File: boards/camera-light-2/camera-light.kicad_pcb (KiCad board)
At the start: 2 copper layers, 10 x 9 mm, 3 parts, among them P1 CONN_01X02

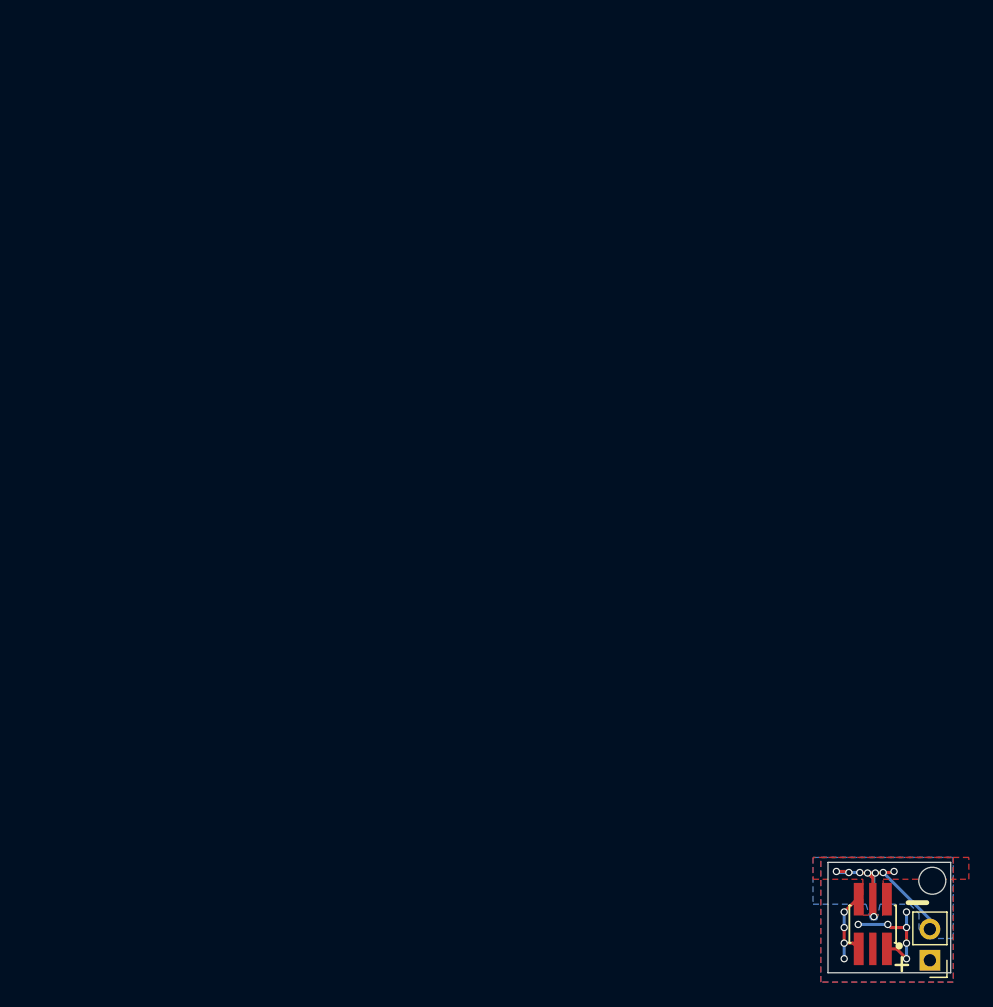
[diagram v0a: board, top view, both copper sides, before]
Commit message: [camera-light-2] export schematic and layout
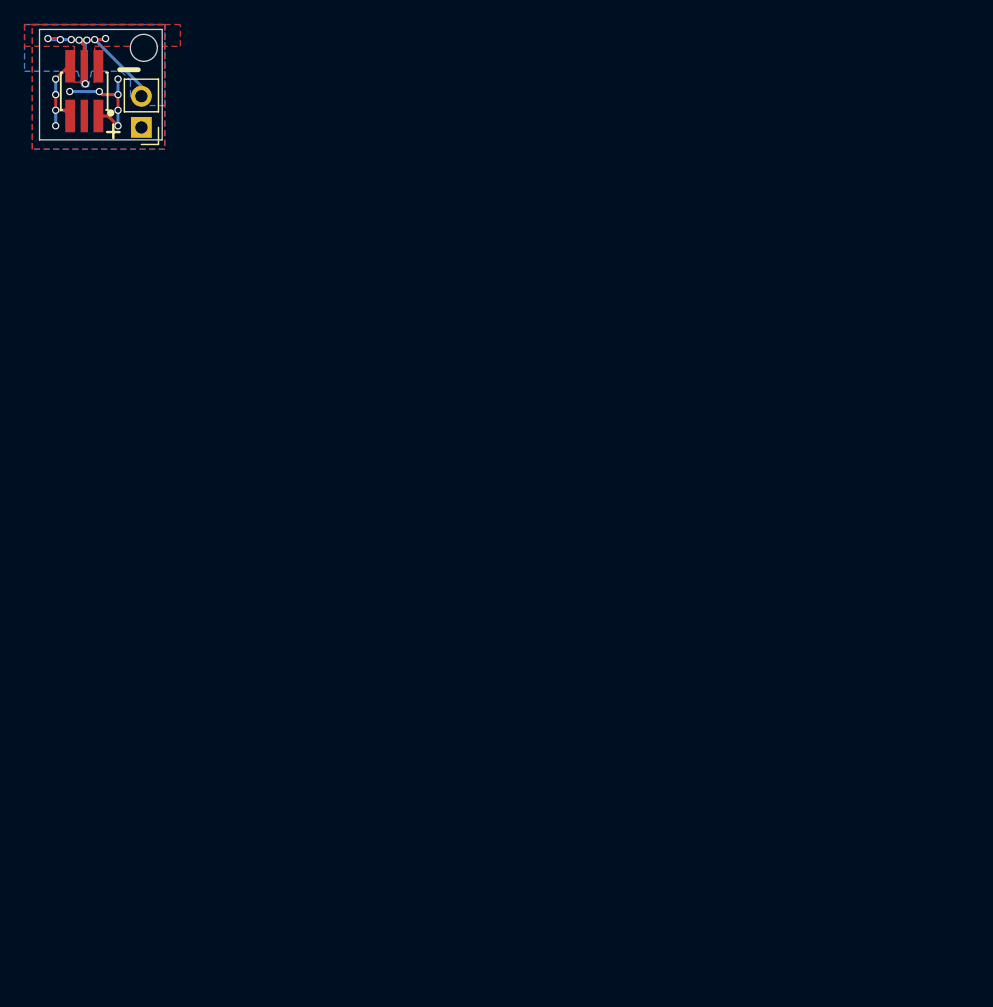
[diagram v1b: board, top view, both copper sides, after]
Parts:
- moved D1 93.5 mm to (84.2, 37.1)
- moved P1 93.5 mm to (90.0, 42.1)
- moved REF** 93.5 mm to (90.2, 35.6)
